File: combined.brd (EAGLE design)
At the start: 179 x 79.7 mm, 201 parts, among them U1 LM4562MAX/NOPB, U10 LM4562MAX/NOPB, U11 LM4562MAX/NOPB, U12 MAX5419LETA+, U13 MAX5419LETA+, U14 LM4562MAX/NOPB, U15 LM4562MAX/NOPB, U16 LM4562MAX/NOPB, U17 LM4562MAX/NOPB, U2 LM4562MAX/NOPB, U3 LM4562MAX/NOPB, U4 LM4562MAX/NOPB, U5 LM4562MAX/NOPB, U6 MAX5419LETA+, U7 MAX5419LETA+, U8 LM4562MAX/NOPB, U9 LM4562MAX/NOPB

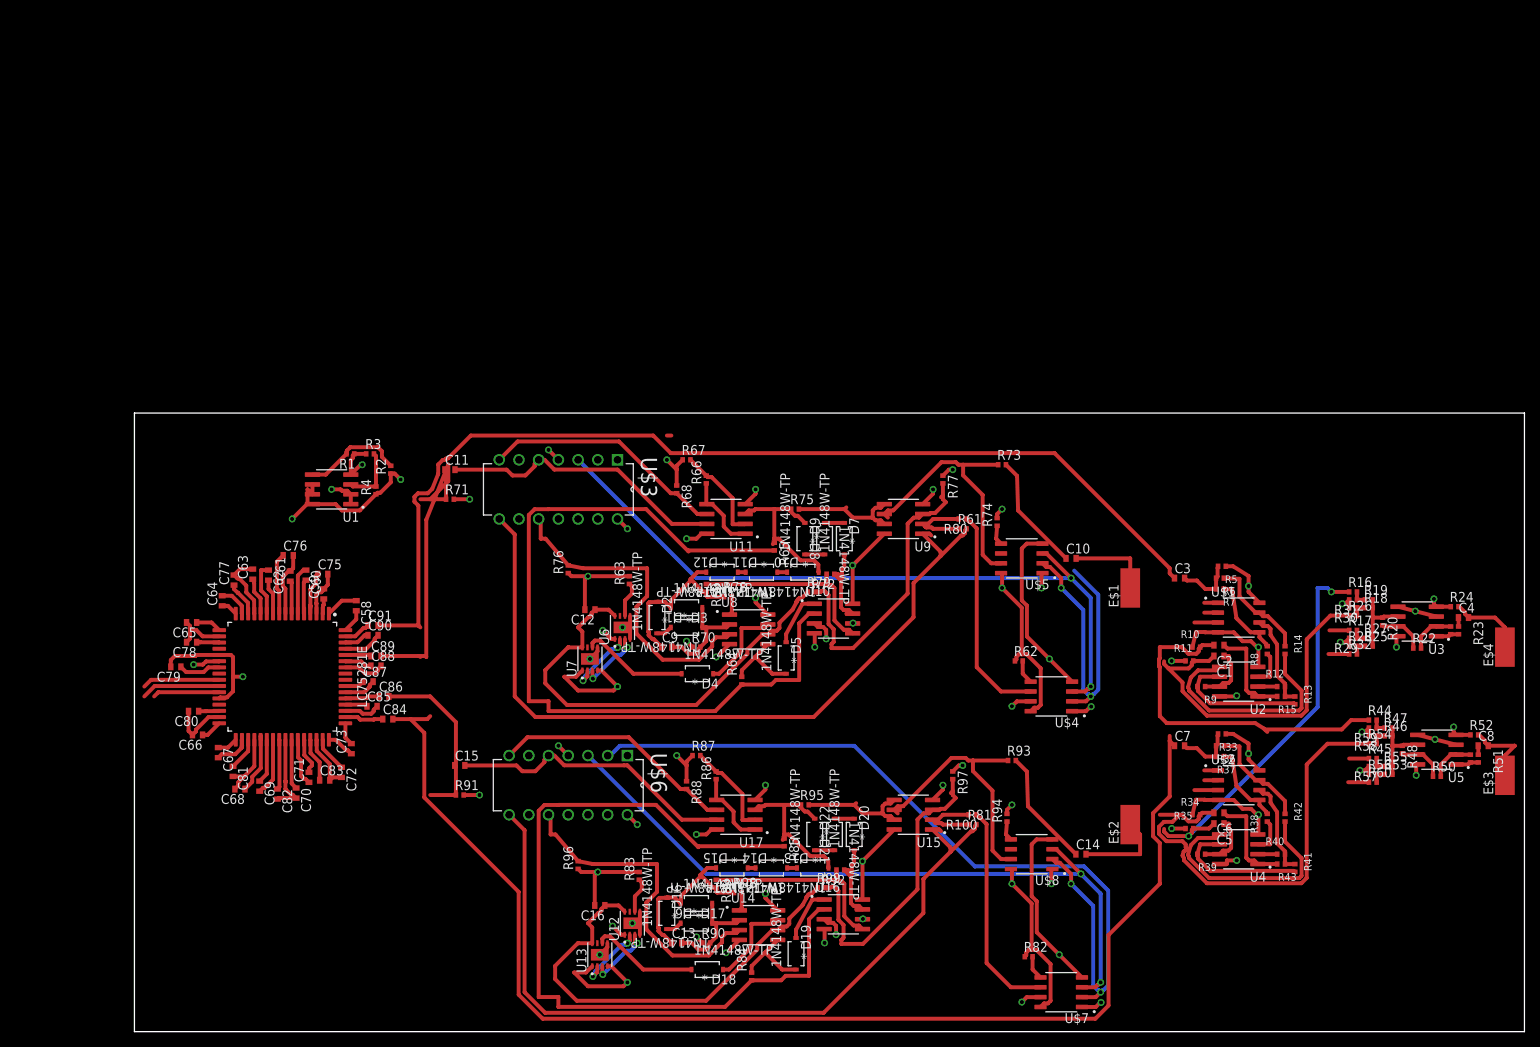
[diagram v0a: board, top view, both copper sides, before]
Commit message: corrections
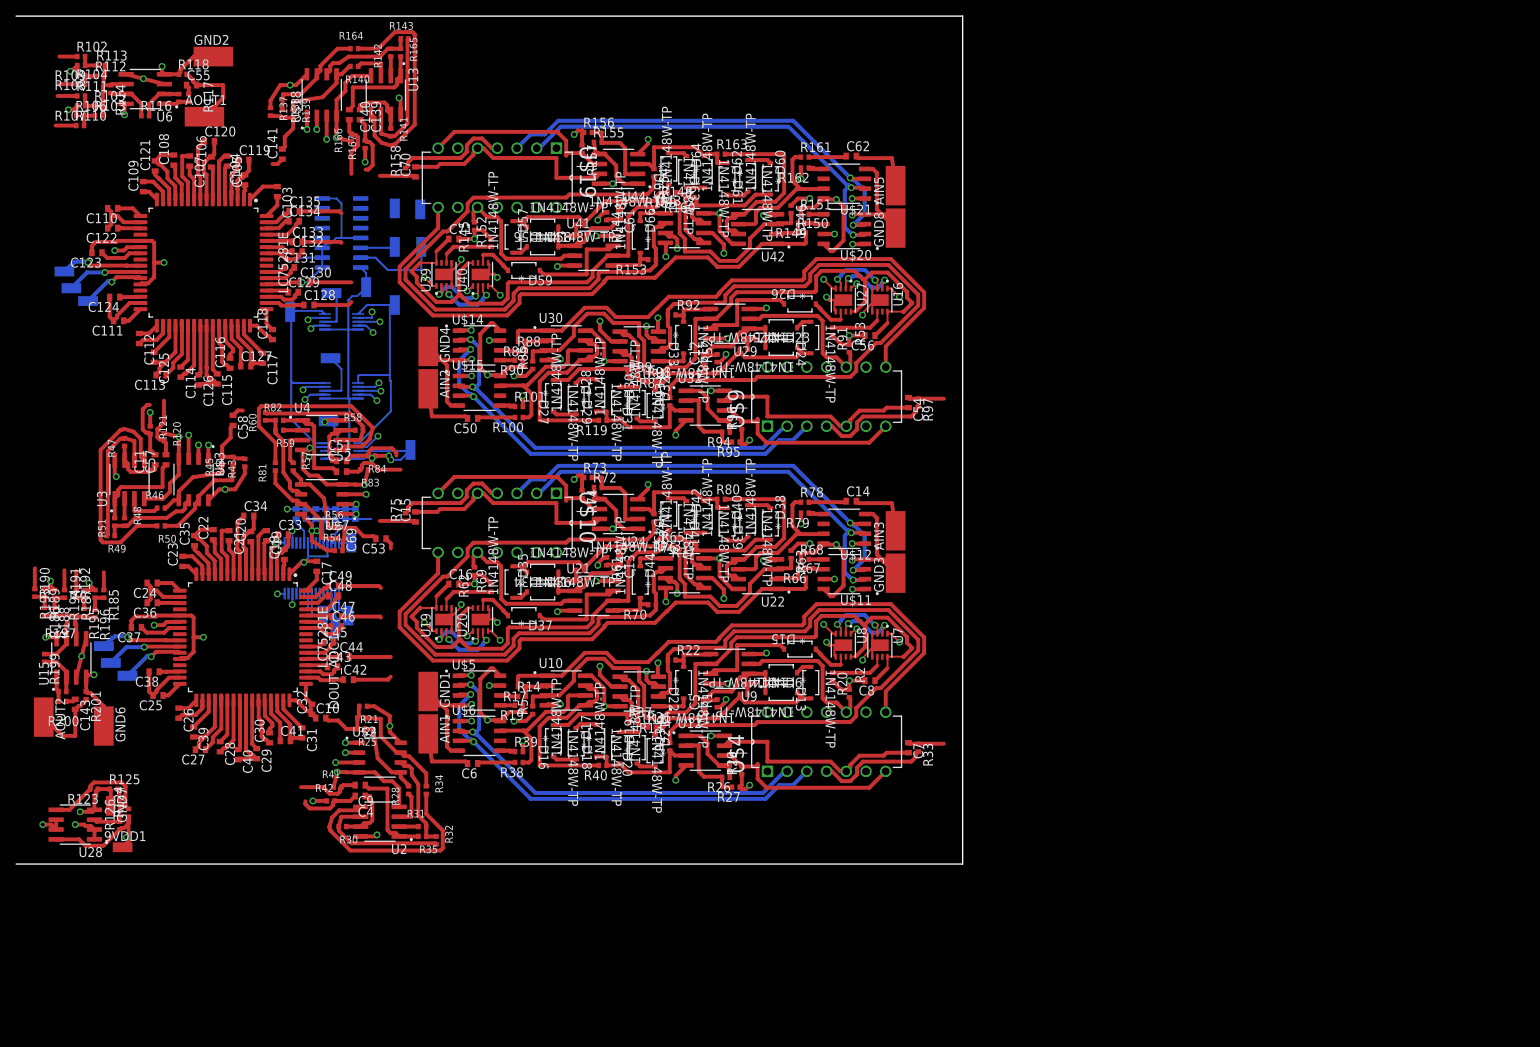
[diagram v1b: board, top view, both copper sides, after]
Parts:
- removed C1, C2, C3: 0.1u, rcl:C0402
- removed C59, C60, C72, C73: 0.047uF, rcl:C0402
- removed C75, C76, C77, C78, C79, C80, C81, C82, C83, C84, C85, C86, C87, C88, C89, C90, C91: 10uF, rcl:C0402
- removed D1, D10, D11, D12, D2, D3, D4, D5, D7, D8, D9: 1N4148W-TP, 1N4148W-TP:SOD123
- removed E$1, E$2, E$3, E$4: (no value), wirepad:SMD2,54-5,08
- removed R10, R11: 1.5M, rcl:R0402
- removed R15, R18, R9: 20k, rcl:R0402
- removed R16: 5k, rcl:R0402
- removed R3: 1k, rcl:R0402
- removed R4: 1.7k, rcl:R0402
- removed R6, R7: 10k, rcl:R0402
- removed R8: 4k, rcl:R0402
- removed U$1, U$8: MCP4131-503E/SN, MCP4131-503E_SN:SOIC127P599X175-8N
- removed U1, U14, U5: LM4562MAX/NOPB, LM4562MAX_NOPB:SOIC127P599X175-8N
- added 3V3_D1, 9VDD1, BCK_ADC1, CE_EQ1, CE_EQ2, CLK_ADC1, CL_EQ1, CL_EQ2, CS3, CS4, CS5, DI_EQ1, DI_EQ2, DOUT_ADC1, GND5, GND7, LRCK_ADC1, MUX2, MUX3, SCK1, SCL1, SDA1, SDI/O1: (no value), wirepad:SMD1,27-2,54
- added AIN1, AIN2, AIN3, AIN5, AOUT1, AOUT2, GND1, GND2, GND3, GND4, GND6, GND8: (no value), wirepad:SMD2,54-5,08
- added C103, C104, C105, C106, C107, C108, C109, C110, C111, C112, C113, C114, C115, C116, C117, C118, C17, C18, C19, C20, C21, C22, C23, C24, C25, C26, C27, C28, C29, C30, C31, C32: 0.047uF, rcl:C0402
- added C119, C120, C121, C122, C123, C124, C125, C126, C127, C128, C129, C130, C131, C132, C133, C134, C135, C33, C34, C35, C36, C37, C38, C39, C40, C41, C42, C43, C44, C45, C46, C47, C48, C49: 10uF, rcl:C0402
- added C139, C140, C141, C143, C51, C52, C53, C55, C57: 0.1u, rcl:C0402
- added C50: 0.1, rcl:C0402
- added C54, C56: 1.5u, rcl:C0402
- added D23, D24, D25, D26, D27, D28, D29, D30, D31, D32, D33, D34, D35, D36, D37, D38, D39, D40, D41, D42, D43, D44, D56, D57, D58, D59, D60, D61, D62, D63, D64, D65, D66: 1N4148W-TP, 1N4148W-TP:SOD123
- added IC2: PCM1865DBT, PCM1865DBT:TSSOP-30
- added R101, R137, R138, R139, R145, R151, R156, R162: 10k, rcl:R0402
- added R102, R104, R106, R107, R108, R109, R110, R111, R185, R187, R189, R190, R191, R192, R193, R194: 5k, rcl:R0402
- added R103, R105, R112, R113, R114, R115, R116, R141, R157, R165, R186, R188, R195, R196, R197, R198, R199: 20k, rcl:R0402
- added R117, R123, R124, R125, R147, R200: 1k, rcl:R0402
- added R118, R120, R121, R166, R167, R201: 1.5M, rcl:R0402
- added R119, R144, R149, R150, R152, R153, R154, R155, R159, R160, R161, R163: 100k, rcl:R0402
- added R126: 1.7k, rcl:R0402
- added R140, R164: 4k, rcl:R0402
- added R142, R143: 6k, rcl:R0402
- added R146, R148: 470k, rcl:R0402
- added R158: 1M, rcl:R0402
- added U$10, U$19, U$9: MCP42100-I/P, MCP42100-I_P:DIP254P762X432-14
- added U$11, U$12, U$15, U$18, U$20, U$21: MCP4131-503E/SN, MCP4131-503E_SN:SOIC127P599X175-8N
- added U$13, U$16: LC75281E, LC75281E:QFP80P1720X1720X270-64N
- added U18, U25: TMUX1204DGSR, TMUX1204DGSR:SOP50P490X110-10N
- added U19, U20, U27, U39, U40: MAX5419LETA+, MAX5419LETA_:SON65P300X300X80-9N
- added U21, U22, U23, U24, U28, U29, U30, U31, U32, U41, U42, U43, U44: LM4562MAX/NOPB, LM4562MAX_NOPB:SOIC127P599X175-8N
- added U26: TCA9546ADR, TCA9546ADR:SOIC127P600X175-16N
- C10: value 0.1 -> 0.1u
- C11: value 1.5u -> 0.1u
- C12: value 1.5u -> 680p
- C5: value 0.1u -> 680p
- C58: value 0.047uF -> 0.1u
- C6: value 0.1u -> 0.1
- C61: value 0.047uF -> 680p
- C62: value 0.047uF -> 0.1
- C63, C65, C68: value 0.047uF -> 0.1μF
- C64, C66: value 0.047uF -> 10μF
- C67, C69: value 0.047uF -> 1μF
- C7, C8: value 0.1u -> 1.5u
- C70, C71: value 0.047uF -> 1.5u
- C9: value 680p -> 0.1u
- R1, R23, R78, R98: value 1k -> 100k
- R12: value 6k -> 1k
- R13: value 6k -> 470k
- R14, R38: value 4k -> 100k
- R17, R26: value 5k -> 100k
- R19, R21, R25, R27, R39, R43, R53, R55, R68: value 20k -> 10k
- R2: value 1k -> 10k
- R20, R22, R88: value 20k -> 100k
- R24: value 1.5M -> 10k
- R28, R57: value 5k -> 4k
- R29, R30, R58: value 5k -> 20k
- R31, R32, R59, R60: value 5k -> 6k
- R33: value 10k -> 1M
- R34: value 1.5M -> 4k
- R35: value 1.5M -> 20k
- R36, R37, R67, R76, R94: value 10k -> 100k
- R40: value 6k -> 100k
- R41: value 6k -> 1.5M
- R42: value 4k -> 1.5M
- R44, R45, R54, R56: value 5k -> 10k
- R46, R50: value 20k -> 4k
- R48, R49: value 20k -> 6k
- R5, R87: value 10k -> 470k
- R51: value 1k -> 20k
- R52: value 1.5M -> 100k
- R63, R65, R85: value 100k -> 470k
- R64, R86: value 100k -> 1k
- R71, R91: value 1M -> 100k
- R73, R90, R95: value 100k -> 10k
- R74, R82, R96: value 10k -> 20k
- R75: value 100k -> 1M
- R77, R99: value 470k -> 100k
- R79: value 470k -> 10k
- R81: value 100k -> 4k
- R83, R84: value 100k -> 1.5M
- R97: value 470k -> 1M
- U$14: value LC75281E -> MCP4131-503E/SN; device LC75281E:QFP80P1720X1720X270-64N -> MCP4131-503E_SN:SOIC127P599X175-8N
- U$3, U$6: value MCP42100-I/P -> MCP4131-503E/SN; device MCP42100-I_P:DIP254P762X432-14 -> MCP4131-503E_SN:SOIC127P599X175-8N
- U$4: value MCP4131-503E/SN -> MCP42100-I/P; device MCP4131-503E_SN:SOIC127P599X175-8N -> MCP42100-I_P:DIP254P762X432-14
- U12, U13, U6: value MAX5419LETA+ -> LM4562MAX/NOPB; device MAX5419LETA_:SON65P300X300X80-9N -> LM4562MAX_NOPB:SOIC127P599X175-8N
- U16, U8: value LM4562MAX/NOPB -> MAX5419LETA+; device LM4562MAX_NOPB:SOIC127P599X175-8N -> MAX5419LETA_:SON65P300X300X80-9N
- U17: value LM4562MAX/NOPB -> TMUX1204DGSR; device LM4562MAX_NOPB:SOIC127P599X175-8N -> TMUX1204DGSR:SOP50P490X110-10N
- moved R51 178.3 mm to (12.7, 44.1)
- moved R49 177.5 mm to (12.2, 42.3), turned to 180 degrees
- moved R50 167.5 mm to (18.7, 43.6), turned to 180 degrees
- moved R48 167.2 mm to (14.0, 44.1)
- moved R47 166.9 mm to (14.0, 54.4), turned to 90 degrees
- moved U3 166.9 mm to (14.6, 49.5), turned to 90 degrees
- moved R46 160.8 mm to (18.7, 45.8)
- moved R45 153.1 mm to (26.5, 51.9), turned to 90 degrees
- moved R44 150.6 mm to (27.9, 51.9), turned to 90 degrees
- moved R60 150.2 mm to (32.1, 57.7), turned to 90 degrees
- moved R59 146.0 mm to (33.9, 55.9)
- moved R57 144.3 mm to (35.7, 51.2), turned to 270 degrees
- moved C4 144.0 mm to (44.3, 8.76), turned to 180 degrees
- moved R43 143.1 mm to (29.5, 51.7), turned to 90 degrees
- moved R24 141.6 mm to (44.5, 18.8), turned to 180 degrees
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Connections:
- removed net CS5: U$7.1
- removed net CS6: U$8.1
- removed net EQ1_CE: U$14.27
- removed net EQ1_CL: U$14.25
- removed net EQ1_DI: U$14.26
- removed net H_1: C16.1, R99.1, U12.8, U13.8, U14.6
- removed net L_2: R83.1, U12.6
- removed net L_3: D18.C, U13.6
- removed net N$12: R21.2, R23.1, U3.1
- removed net N$123: C58.1, U$14.1
- removed net N$125: C60.1, U$14.6
- removed net N$126: C61.1, U$14.7
- removed net N$127: C62.1, U$14.11
- removed net N$128: C63.1, U$14.12
- removed net N$129: C64.1, U$14.16
- removed net N$130: C65.1, U$14.17
- removed net N$134: C67.1, U$14.33
- removed net N$180: C68.1, U$14.37
- removed net N$183: C71.1, U$14.43
- removed net N$184: C72.1, U$14.47
- removed net N$185: C73.1, U$14.48
- removed net N$186: C58.2, U$14.64
- removed net N$187: C59.2, C75.2, U$14.3
- removed net N$188: C75.1, U$14.4
- removed net N$189: C76.1, U$14.9
- removed net N$190: C77.1, U$14.14
- removed net N$192: C79.1, U$14.23
- removed net N$193: C80.1, U$14.30
- removed net N$194: C81.1, U$14.35
- removed net N$195: C82.1, U$14.40
- removed net N$196: C83.1, U$14.45
- removed net N$197: C84.1, U$14.50
- removed net N$198: C85.1, U$14.52
- removed net N$199: C86.1, U$14.53
- removed net N$200: C87.1, U$14.55
- removed net N$201: C88.1, U$14.59
- removed net N$202: C89.1, U$14.60
- removed net N$203: C90.1, U$14.62
- removed net N$204: C91.1, U$14.63
- removed net N$205: C60.2, U$14.5
- removed net N$206: C61.2, C76.2, U$14.8
- removed net N$207: C62.2, U$14.10
- removed net N$208: C63.2, C77.2, U$14.13
- removed net N$209: C64.2, U$14.15
- removed net N$210: C65.2, C78.2, U$14.18
- removed net N$212: C67.2, U$14.34
- removed net N$214: C69.2, U$14.39
- removed net N$215: C70.2, C82.2, U$14.41
- removed net N$216: C71.2, U$14.44
- removed net N$217: C72.2, C83.2, U$14.46
- removed net N$218: C73.2, U$14.49
- removed net N$219: C85.2, U$14.51
- removed net N$222: C88.2, U$14.58
- removed net N$224: C90.2, U$14.61
- removed net N$24: R42.2, U4.5
- removed net N$25: R38.1, U4.3
- removed net N$32: R46.2, R47.2, R48.1, R53.2, R55.2, U5.6
- removed net N$5 (its old number): R8.1, U2.3
- removed net P0A_2: R82.2, U$7.5
- removed net P0A_3: R94.1, U$8.5
- removed net P0B_2: R93.1, U$8.7, U15.6
- removed net P0W_1: R100.1, U$7.6
- removed net PA2: R81.2, U$6.8, U15.1
- removed net PA3: R88.2, U$6.7, U17.6
- removed net PB2: R96.2, U$6.10, U14.3
- removed net PB3: C15.2, U$6.5, U17.7
- removed net S$1: U$4.2, U$5.2
- removed net S$2: U$3.2
- removed net S$4: U1.6, U1.7
- removed net S$5: R2.1, R4.1, U1.8
- removed net SCK1: U$2.2
- removed net SCK2: U$6.2, U$7.2, U$8.2
- removed net SCL1: U12.2, U13.2
- removed net SDA1: U12.3, U13.3
- removed net SDI/O1: U$2.3
- removed net SDI/O2: U$3.3, U$4.3, U$5.3
- removed net SDI/O3: U$6.3, U$7.3, U$8.3
- removed net VDD1: R62.1, U$3.14, U$4.8, U$5.8, U10.8, U11.8, U6.1, U7.1, U7.4, U8.8, U9.8
- removed net VDD2: R82.1, U$6.14, U$7.8, U$8.8, U12.1, U13.1, U13.4, U14.8, U15.8, U16.8, U17.8
- removed net VREF1: C12.2, R63.2, R67.1, R68.1, R70.1, R74.2, R76.1, R77.1, U$4.7, U10.3, U10.6
- removed net VREF2: C16.2, R83.2, R87.1, R88.1, R90.1, R94.2, R96.1, R97.1, U$7.7, U16.3, U16.6
- removed net VSS1: R91.2, U$6.4, U$7.4, U$8.4, U12.4, U12.5, U12.9, U13.5, U13.9, U14.4, U15.4, U16.4, U17.4
- new net +3V3: 3V3_D1.1, U17.5, U17.6, U18.5, U18.6, U25.5, U25.6, U26.16
- new net 3V3D: C63.1, C64.1, IC2.13, IC2.14
- new net AIN01: R110.1
- new net AIN02: R193.1
- new net AIN11: R111.1
- new net AIN12: C53.1
- new net AIN123: R194.1
- new net AIN223: R187.1
- new net AIN31: C141.1
- new net AIN323: R185.1
- new net AIN33: AIN2.1, C50.2
- new net AIN45: C58.1
- new net AOUT2: C15.1, R75.1
- new net AOUT23: AOUT2.1, C143.2, R201.2
- new net AOUT3: C54.1, R97.1
- new net AOUT4: C70.1, R158.1
- new net AOUTL3: C140.2, R166.2
- new net AOUTL4: C57.2, R120.2
- new net AOUTR3: C139.2, R167.2
- new net AOUTR4: C11.2, R121.2
- new net BCK_ADC: BCK_ADC1.1, IC2.17
- new net CLK_ADC: CLK_ADC1.1, IC2.15
- new net CS01: U$10.1
- new net CS03: U$9.1
- new net CS04: U$19.1
- new net CS0D: CS3.1, U17.8
- new net CS0_0: U17.2
- new net CS0_1: U17.9
- new net CS0_2: U17.4
- new net CS0_3: U17.7
- new net CS11: U$11.1
- new net CS13: U$14.1
- new net CS14: U$20.1
- new net CS1D: CS4.1, U25.8
- new net CS1_0: U25.2
- new net CS1_1: U25.9
- new net CS1_2: U25.4
- new net CS1_3: U25.7
- new net CS21: U$12.1
- new net CS23: U$15.1
- new net CS24: U$21.1
- new net CS2D: CS5.1, U18.8
- new net CS2_0: U18.2
- new net CS2_1: U18.9
- new net CS2_2: U18.4
- new net CS2_3: U18.7
- new net DGND: GND5.1, U17.3, U18.3, U25.3, U26.1, U26.13, U26.2, U26.3, U26.8
- new net DOUT_ADC: DOUT_ADC1.1, IC2.18
- new net EIN01: C130.2
- new net EIN11: C133.2
- new net EOUT01: C128.2
- new net EOUT11: C135.2
- new net EQ1_CE1: CE_EQ1.1, U$13.27
- new net EQ1_CE2: CE_EQ2.1, U$16.27
- new net EQ1_CL1: CL_EQ1.1, U$13.25
- new net EQ1_CL2: CL_EQ2.1, U$16.25
- new net EQ1_DI1: DI_EQ1.1, U$13.26
- new net EQ1_DI2: DI_EQ2.1, U$16.26
- new net H_01: C16.1, R65.1, U19.8, U20.8, U21.6
- new net H_03: C56.1, R87.1, U16.8, U27.8, U29.6
- new net H_04: C71.1, R148.1, U39.8, U40.8, U41.6
- new net LRCK_ADC: IC2.16, LRCK_ADC1.1
- new net L_01: R69.1, U19.6
- new net L_03: R91.1, U16.6
- new net L_04: R152.1, U39.6
- new net L_11: D37.C, U20.6
- new net L_13: D26.C, U27.6
- new net L_14: D59.C, U40.6
- new net MUX0: MUX2.1, U17.1, U18.1, U25.1
- new net MUX1: MUX3.1, U17.10, U18.10, U25.10
- new net N$100: C105.1, U$16.6
- new net N$101: C106.1, U$16.7
- new net N$102: D56.A, D57.C
- new net N$103: D61.A, D62.C
- new net N$104: D60.A, D61.C
- new net N$105: C62.1, R161.2
- new net N$106: D64.A, D65.C
- new net N$107: D63.A, D64.C
- new net N$108: C107.1, U$16.11
- new net N$109: C108.1, U$16.12
- new net N$110: C109.1, U$16.16
- new net N$111: C110.1, U$16.17
- new net N$112: C111.1, U$16.32
- new net N$113: C112.1, U$16.33
- new net N$114: C113.1, U$16.37
- new net N$115: C114.1, U$16.38
- new net N$116: C115.1, U$16.42
- new net N$117: C116.1, U$16.43
- new net N$118: C117.1, U$16.47
- new net N$119: C118.1, U$16.48
- new net N$120: C103.2, U$16.64
- new net N$121: C104.2, C119.2, U$16.3
- new net N$122: C119.1, U$16.4
- new net N$124: C120.1, U$16.9
- new net N$131: C121.1, U$16.14
- new net N$132: C122.1, U$16.19
- new net N$135: C123.1, U$16.23
- new net N$136: C124.1, U$16.30
- new net N$137: C125.1, U$16.35
- new net N$138: C126.1, U$16.40
- new net N$139: C127.1, U$16.45
- new net N$140: C128.1, U$16.50
- new net N$141: D37.A, U21.7
- new net N$1413: R103.2, R105.2, R112.2, R113.2, R114.1, U6.6
- new net N$142: D39.A, D40.C
- new net N$1421: R186.2, R188.2, R195.2, R196.2, R197.1, U15.6
- new net N$143: C129.1, U$16.52
- new net N$1433: D26.A, U29.7
- new net N$144: R147.2, U41.1
- new net N$1444: D59.A, U41.7
- new net N$145: C130.1, U$16.53
- new net N$146: C131.1, U$16.55
- new net N$147: C132.1, U$16.59
- new net N$148: C133.1, U$16.60
- new net N$149: C134.1, U$16.62
- new net N$150: C135.1, U$16.63
- new net N$151: D44.C, R70.2, U21.5
- new net N$152: D38.A, D39.C
- new net N$153: C105.2, U$16.5
- new net N$1533: D33.C, R92.2, U29.5
- new net N$154: C106.2, C120.2, U$16.8
- new net N$1544: D66.C, R153.2, U41.5
- new net N$155: C107.2, U$16.10
- new net N$156: C108.2, C121.2, U$16.13
- new net N$157: C109.2, U$16.15
- new net N$158: C110.2, C122.2, U$16.18
- new net N$159: C111.2, C124.2, U$16.31
- new net N$160: C112.2, U$16.34
- new net N$161: R70.1, R71.2, U23.2
- new net N$162: C14.1, R78.2
- new net N$163: C113.2, C125.2, U$16.36
- new net N$1633: R92.1, R93.2, U31.2
- new net N$164: C114.2, U$16.39
- new net N$1644: R153.1, R154.2, U43.2
- new net N$165: C115.2, C126.2, U$16.41
- new net N$166: C116.2, U$16.44
- new net N$167: C117.2, C127.2, U$16.46
- new net N$168: C118.2, U$16.49
- new net N$169: C129.2, U$16.51
- new net N$170: C131.2, U$16.54
- new net N$171: C132.2, U$16.58
- new net N$172: C134.2, U$16.61
- new net N$173: C104.1, U$16.2
- new net N$175: C141.2, R137.2, R138.2, R139.2
- new net N$1833: R94.1, U32.1, U32.5
- new net N$1844: R155.1, U44.1, U44.5
- new net N$1933: R94.2, R95.2, U32.2
- new net N$1944: R155.2, R156.2, U44.2
- new net N$2012: C53.2, R54.2, R55.2, R56.2
- new net N$2111: C13.1, D35.A, D36.C, D43.A, R64.1, R76.2
- new net N$21111: C17.1, U$13.1
- new net N$2133: C12.1, D24.A, D25.C, D32.A, R86.1, R98.2
- new net N$2144: C61.1, D57.A, D58.C, D65.A, R147.1, R159.2
- new net N$223: C143.1, R200.2
- new net N$225: R186.1, R189.2, R193.2
- new net N$226: R185.2, R192.1, R196.1
- new net N$227: R187.2, R191.1, R195.1
- new net N$228: R188.1, R190.1, R194.2
- new net N$233: D27.C, R99.1, U31.7
- new net N$244: D60.C, R160.1, U43.7
- new net N$246: D62.A, D63.C, R154.1, R163.1, U44.3
- new net N$261: D40.A, D41.C, R71.1, R80.1, U24.3
- new net N$2611: C21.1, U$13.11
- new net N$2633: D29.A, D30.C, R119.1, R93.1, U32.3
- new net N$271: R80.2, U22.5, U22.7
- new net N$2711: C22.1, U$13.12
- new net N$2733: R119.2, U30.5, U30.7
- new net N$2744: R163.2, U42.5, U42.7
- new net N$312: R81.2, U4.5
- new net N$331: R164.2, U13.5
- new net N$333: C12.2, D23.C, D25.A, R52.2, U29.2
- new net N$344: C61.2, D56.C, D58.A, R144.2, U41.2
- new net N$411: C17.2, U$13.64
- new net N$413: R114.2, R116.1, U6.7
- new net N$414: R50.2, U3.5
- new net N$421: R197.2, R199.1, U15.7
- new net N$433: D33.A, U31.1
- new net N$444: D66.A, U43.1
- new net N$500: R28.1, U2.3
- new net N$512: R57.1, U4.3
- new net N$513: R115.1, R116.2, U6.2
- new net N$514: R46.1, U3.3
- new net N$521: R198.1, R199.2, U15.2
- new net N$531: R140.1, U13.3
- new net N$600: R31.1, U2.2
- new net N$611: C20.2, C34.2, U$13.8
- new net N$612: R59.1, U4.2
- new net N$614: R48.1, U3.2
- new net N$631: R142.1, U13.2
- new net N$633: R85.2, R87.2, U30.3
- new net N$644: R146.2, R148.2, U42.3
- new net N$68: C27.2, C39.2, U$13.36
- new net N$700: R30.2, R32.2, U2.6
- new net N$711: C30.2, U$13.44
- new net N$712: R58.2, R60.2, U4.6
- new net N$714: R47.2, R49.2, U3.6
- new net N$731: R141.2, R143.2, U13.6
- new net N$733: R88.2, R89.1, U30.2
- new net N$744: R149.2, R150.1, U42.2
- new net N$78: C18.1, U$13.2
- new net N$80: C55.1, R117.2
- new net N$800: C4.1, R30.1, U2.7
- new net N$81: R76.1, R77.2, U23.5
- new net N$812: C51.1, R58.1, U4.7
- new net N$814: C11.1, R47.1, U3.7
- new net N$82: R103.1, R106.2, R110.2
- new net N$83: R102.2, R109.1, R113.1
- new net N$831: C139.1, R141.1, U13.7
- new net N$833: R98.1, R99.2, U31.5
- new net N$84: R104.2, R108.1, R112.1
- new net N$844: R159.1, R160.2, U43.5
- new net N$85: R105.1, R107.1, R111.2
- new net N$86: D23.A, D24.C
- new net N$87: D28.A, D29.C
- new net N$88: C67.1, IC2.6
- new net N$89: C68.1, C69.1, IC2.11
- new net N$90: D27.A, D28.C
- new net N$91: C50.1, R100.2
- new net N$912: C52.1, R82.2, U4.1
- new net N$914: C57.1, R51.2, U3.1
- new net N$92: R125.2, R126.2, U28.3
- new net N$93: R123.2, R124.2, U28.5
- new net N$931: C140.1, R165.2, U13.1
- new net N$94: D31.A, D32.C
- new net N$95: D30.A, D31.C
- new net N$99: C103.1, U$16.1
- new net P0A31: R139.1, R140.2, U$18.5
- new net P0A4: R45.1, R46.2, U$3.5
- new net P0A_01: R68.2, U$11.5
- new net P0A_03: R90.2, U$14.5
- new net P0A_04: R151.2, U$20.5
- new net P0A_11: R79.1, U$12.5
- new net P0A_13: R101.1, U$15.5
- new net P0A_14: R162.1, U$21.5
- new net P0B31: R138.1, R164.1, U$18.7
- new net P0B4: R44.1, R50.1, U$3.7
- new net P0B_11: R78.1, U$12.7, U22.6
- new net P0B_13: R100.1, U$15.7, U30.6
- new net P0B_14: R161.1, U$21.7, U42.6
- new net P0W31: R142.2, R143.1, R165.1, U$18.6
- new net P0W4: R48.2, R49.1, R51.1, U$3.6
- new net P0W_01: R66.1, U$11.6
- new net P0W_03: R88.1, U$14.6
- new net P0W_04: R149.1, U$20.6
- new net PA01: R67.2, U$10.8, U22.1
- new net PA03: R89.2, U$9.8, U30.1
- new net PA04: R150.2, U$19.8, U42.1
- new net PA11: R74.2, U$10.7, U24.6
- new net PA13: R96.2, U$9.7, U32.6
- new net PA14: R157.2, U$19.7, U44.6
- new net PB01: R62.2, U$10.10, U21.3
- new net PB03: R53.2, U$9.10, U29.3
- new net PB04: R145.2, U$19.10, U41.3
- new net PB11: C15.2, U$10.5, U24.7
- new net PB13: C54.2, U$9.5, U32.7
- new net PB14: C70.2, U$19.5, U44.7
- new net RS3: U$9.11
- new net RS4: U$19.11
- new net SCL_0: U26.5
- new net SCL_1: U26.4
- new net SCL_2: U26.10
- new net SCL_3: U26.9
- new net SDA_0: U26.7
- new net SDA_1: U26.6
- new net SDA_2: U26.12
- new net SDA_3: U26.11
- new net SHDN3: U$9.12
- new net SHDN4: U$19.12
- new net VIN1: IC2.1
- new net VIN2: IC2.3
- new net VIN3: IC2.30
- new net VIN4: IC2.28
- net 3V3A: now also C65.1, C66.1, IC2.8, U28.1, U28.2; no longer U1.1, U1.2
- net AIN: now also AIN1.1, C6.2; no longer C10.2, E$1.1
- net AIN0: now also C10.1; no longer R32.1
- net AIN1: now also AIN3.1, C14.2; no longer R17.1
- net AIN2: now also R104.1; no longer C14.2, E$2.1
- net AIN3: now also R102.1; no longer R60.1
- net AIN4: now also AIN5.1, C62.2; no longer R45.1
- net AOUT: now also C7.1, R33.1; no longer C4.2, E$4.1, R24.2
- net AOUT1: now also AOUT1.1, C55.2, R118.2; no longer C8.2, E$3.1, R52.2
- net AOUTL: now also C9.2, R41.2; no longer C2.2, R10.2, R44.1
- net AOUTL1: now also C52.2, R83.2; no longer C6.2, R34.2, R54.1
- net AOUTR: now also C4.2, R42.2; no longer C1.2, R11.2, R26.1
- net AOUTR1: now also C51.2, R84.2; no longer C5.2, R16.1, R35.2
- net CS: now also U$2.1; no longer U$1.1
- net CS0: now also U$4.1; no longer U$3.1
- net CS1: now also U$5.1, U$7.1; no longer U$2.1
- net CS2: now also U$6.1; no longer U$4.1
- net CS3: now also U$18.1; no longer U$5.1
- net CS4: now also U$3.1; no longer U$6.1
- net EIN0: now also C44.2; no longer C15.1, C86.2, R91.1
- net EIN1: now also C47.2; no longer C11.1, C89.2, R71.1
- net EOUT0: now also C42.2; no longer C7.1, C84.2
- net EOUT1: now also C49.2; no longer C3.1, C91.2
- net GND: now also C123.2, C37.2, C63.2, C64.2, C65.2, C66.2, C67.2, C68.2, C69.2, GND2.1, GND6.1, GND7.1, IC2.12, IC2.7, R118.1, R120.1, R121.1, R123.1, R125.1, R166.1, R167.1, R201.1, R41.1, R42.1, R83.1, R84.1, U$13.21, U$13.28, U$16.21, U$16.28, U$18.4, U$3.4, U$7.4, U13.4, U15.4, U28.4, U6.4; no longer C79.2, R1.1, R10.1, R11.1, R24.1, R3.1, R34.1, R35.1, R52.1, U$1.4, U$14.21, U$14.28, U1.4, U5.4
- net H_0: now also C8.1, R13.1, U8.8, U9.6; no longer C12.1, R79.1, U6.8, U8.6
- net L_0: now also R20.1, U7.6; no longer R63.1, U6.6
- net L_1: now also D15.C, U8.6; no longer D4.C, U7.6
- net N$1: now also D13.C, D6.A, R12.2, U9.1; no longer R3.2, R4.2, U1.3
- net N$10: now also C10.2, R21.2, R24.2, R25.2; no longer C59.1, U$14.2
- net N$11: now also R64.2, U21.1; no longer C4.1, R23.2
- net N$13: now also D34.A, D35.C; no longer R20.2, R22.1, U3.7
- net N$133: now also R86.2, U29.1; no longer C66.1, U$14.32
- net N$14: now also D15.A, U9.7; no longer R21.1, R22.2, U3.2
- net N$15: now also D22.C, R22.2, U9.5; no longer R25.1, R28.2, R32.2
- net N$16: now also R22.1, R23.2, U11.2; no longer R18.2, R19.2, R20.1, R25.2, R27.2, U3.6
- net N$17: now also D42.A, D43.C; no longer R16.2, R19.1, R31.1
- net N$18: now also R26.1, U12.1, U12.5; no longer R18.1, R26.2, R30.1
- net N$181: now also R72.1, U24.1, U24.5; no longer C69.1, U$14.38
- net N$182: now also D41.A, D42.C; no longer C70.1, U$14.42
- net N$19: now also R26.2, R27.2, U12.2; no longer R17.2, R27.1, R29.1
- net N$191: now also R72.2, R73.2, U24.2; no longer C78.1, U$14.19
- net N$2: now also D16.C, D17.A, D18.C, R37.1, U11.7; no longer R1.2, R2.2, U1.5
- net N$20: now also C58.2, R43.2, R44.2, R45.2; no longer C7.2, R33.2, R36.2, R37.2
- net N$21: now also C5.1, D13.A, D14.C, D21.A, R12.1, R36.2; no longer R39.2, R41.2, U4.6
- net N$211: now also D38.C, R77.1, U23.7; no longer C66.2, C80.2, U$14.31
- net N$213: now also R115.2, R117.1, U6.1; no longer C68.2, C81.2, U$14.36
- net N$22: now also C19.1, U$13.6; no longer C5.1, R39.1, U4.7
- net N$221: now also R198.2, R200.1, U15.1; no longer C87.2, U$14.54
- net N$23: now also C20.1, U$13.7; no longer C6.1, R43.2, U4.1
- net N$26: now also D18.A, D19.C, R23.1, U12.3; no longer U4.2
- net N$27: now also R40.2, U10.5, U10.7; no longer C8.1, R51.2
- net N$28: now also C23.1, U$13.16; no longer R49.2, R51.1, U5.1
- net N$29: now also C24.1, U$13.17; no longer R48.2, R50.1, U5.7
- net N$3: now also C5.2, D14.A, D16.A, D17.C, D6.C, R1.2, U9.2; no longer C3.2, R5.2, R6.2, R7.2
- net N$30: now also R34.2, U2.5; no longer R49.1, R50.2, U5.2
- net N$31: now also C13.2, D34.C, D36.A, R61.2, U21.2; no longer R53.1, R56.2, R60.2
- net N$33: now also C25.1, U$13.32; no longer R44.2, R47.1, R59.1
- net N$34: now also C26.1, U$13.33; no longer R46.1, R54.2, R58.1
- net N$35: now also C27.1, U$13.37; no longer R45.2, R55.1, R57.1
- net N$36: now also C28.1, U$13.38; no longer C9.2, D1.C, D3.A, R70.2, U8.2
- net N$37: now also C29.1, U$13.42; no longer R77.2, R79.2, U9.3
- net N$38: now also C30.1, U$13.43; no longer R61.1, R80.2, U9.2
- net N$39: now also C31.1, U$13.47; no longer D5.C, R64.2, U8.5
- net N$4: now also C6.1, D22.A, R38.2, U11.1; no longer R14.2, U2.5
- net N$40: now also C32.1, U$13.48; no longer R64.1, R65.2, U10.2
- net N$41: now also D44.A, U23.1; no longer R66.1, U11.1, U11.5
- net N$42: now also C18.2, C33.2, U$13.3; no longer R66.2, R67.2, U11.2
- net N$43: now also C33.1, U$13.4; no longer D1.A, D2.C
- net N$44: now also C34.1, U$13.9; no longer C9.1, D12.A, D2.A, D3.C, R69.2, R78.1
- net N$45: now also C35.1, U$13.14; no longer D4.A, U8.7
- net N$46: now also C36.1, U$13.19; no longer D8.A, D9.C
- net N$47: now also C37.1, U$13.23; no longer D7.A, D8.C
- net N$48: now also C38.1, U$13.30; no longer D10.C, D9.A, R65.1, R75.1, U11.3
- net N$49: now also C39.1, U$13.35; no longer R75.2, U9.5, U9.7
- net N$50: now also C40.1, U$13.40; no longer C10.1, R73.2
- net N$51: now also C41.1, U$13.45; no longer D11.A, D12.C
- net N$52: now also C42.1, U$13.50; no longer D10.A, D11.C
- net N$53: now also C43.1, U$13.52; no longer R69.1, R72.2, U10.5
- net N$54: now also C44.1, U$13.53; no longer R78.2, U8.1
- net N$55: now also C45.1, U$13.55; no longer D7.C, R72.1, U10.7
- net N$56: now also C46.1, U$13.59; no longer D5.A, U10.1
- net N$57: now also C47.1, U$13.60; no longer C13.2, D17.A, D6.C, R90.2, U14.2
- net N$58: now also C48.1, U$13.62; no longer R97.2, R99.2, U15.3
- net N$59: now also C49.1, U$13.63; no longer R100.2, R81.1, U15.2
- net N$6: now also D19.A, D20.C, R13.2, R5.2, U10.3; no longer R12.1, U2.2
- net N$60: now also C19.2, U$13.5; no longer D19.C, R84.2, U14.5
- net N$61: now also R63.2, R65.2, U22.3; no longer R84.1, R85.2, U16.2
- net N$62: now also C21.2, U$13.10; no longer R86.1, U17.1, U17.5
- net N$63: now also C22.2, C35.2, U$13.13; no longer R86.2, R87.2, U17.2
- net N$64: now also C23.2, U$13.15; no longer D16.C, D6.A
- net N$65: now also C24.2, C36.2, U$13.18; no longer C13.1, D15.A, D16.A, D17.C, R89.2, R98.1
- net N$66: now also C25.2, C38.2, U$13.31; no longer D18.A, U14.7
- net N$67: now also C26.2, U$13.34; no longer D21.A, D22.C
- net N$69: now also C28.2, U$13.39; no longer D13.C, D22.A, R85.1, R95.1, U17.3
- net N$7: now also R14.2, R17.1, U10.2; no longer R13.2, R9.2, U2.6
- net N$70: now also C29.2, C40.2, U$13.41; no longer R95.2, U15.5, U15.7
- net N$71: now also R66.2, R67.1, U22.2; no longer C14.1, R93.2
- net N$72: now also C31.2, C41.2, U$13.46; no longer D14.A, D15.C
- net N$73: now also C32.2, U$13.49; no longer D13.A, D14.C
- net N$74: now also C43.2, U$13.51; no longer R89.1, R92.2, U16.5
- net N$75: now also C45.2, U$13.54; no longer R98.2, U14.1
- net N$76: now also C46.2, U$13.58; no longer D20.C, R92.1, U16.7
- net N$77: now also C48.2, U$13.61; no longer D19.A, U16.1
- net N$8: now also R36.1, R37.2, U11.5; no longer C1.1, R9.1, U2.7
- net N$9: now also C9.1, R35.2; no longer C2.1, R15.2
- net P0A: now also R25.1, R28.2, U$2.5; no longer R7.1, R8.2, U$1.5
- net P0A1: now also R56.1, R57.2, U$7.5; no longer R37.1, R38.2, U$2.5
- net P0A_0: now also R19.2, U$5.5; no longer R62.2, U$4.5
- net P0A_1: now also R39.1, U$6.5; no longer R74.1, U$5.5
- net P0B: now also R24.1, R34.1, U$2.7; no longer R14.1, R6.1, U$1.7
- net P0B1: now also R55.1, R81.1, U$7.7; no longer R36.1, R42.1, U$2.7
- net P0B_1: now also R38.1, U$6.7, U10.6; no longer R73.1, U$5.7, U9.6
- net P0W: now also R31.2, R32.1, R35.1, U$2.6; no longer R12.2, R13.1, R15.1, U$1.6
- net P0W1: now also R59.2, R60.1, R82.1, U$7.6; no longer R40.2, R41.1, R43.1, U$2.6
- net P0W_0: now also R14.1, U$5.6; no longer R80.1, U$4.6
- net PA0: now also R17.2, U$4.8, U10.1; no longer R61.2, U$3.8, U9.1
- net PA1: now also R29.2, U$4.7, U12.6; no longer R68.2, U$3.7, U11.6
- net PB0: now also R2.2, U$4.10, U9.3; no longer R76.2, U$3.10, U8.3
- net PB1: now also C7.2, U$4.5, U12.7; no longer C11.2, U$3.5, U11.7
- net RS: now also U$4.11; no longer U$3.11
- net RS1: now also U$10.11; no longer U$6.11
- net SCK: now also SCK1.1, U$10.2, U$11.2, U$12.2, U$14.2, U$15.2, U$18.2, U$19.2, U$2.2, U$20.2, U$21.2, U$3.2, U$4.2, U$5.2, U$6.2, U$7.2, U$9.2; no longer U$1.2
- net SCL: now also IC2.24, SCL1.1, U16.2, U19.2, U20.2, U26.14, U27.2, U39.2, U40.2, U8.2; no longer U6.2
- net SDA: now also IC2.23, SDA1.1, U16.3, U19.3, U20.3, U26.15, U27.3, U39.3, U40.3, U8.3; no longer U6.3
- net SDI/O: now also SDI/O1.1, U$10.3, U$11.3, U$12.3, U$14.3, U$15.3, U$18.3, U$19.3, U$2.3, U$20.3, U$21.3, U$3.3, U$4.3, U$5.3, U$6.3, U$7.3, U$9.3; no longer U$1.3
- net SHDN: now also U$4.12; no longer U$3.12
- net SHDN1: now also U$10.12; no longer U$6.12
- net VDD: now also 9VDD1.1, R124.1, R126.1, R151.1, R19.1, R68.1, R90.1, U$10.14, U$11.8, U$12.8, U$13.22, U$14.8, U$15.8, U$16.22, U$19.14, U$20.8, U$21.8, U$4.14, U$5.8, U$6.8, U$9.14, U10.8, U11.8, U12.8, U13.8, U15.8, U16.1, U19.1, U20.1, U20.4, U21.8, U22.8, U23.8, U24.8, U27.1, U27.4, U28.8, U29.8, U30.8, U31.8, U32.8, U39.1, U40.1, U40.4, U41.8, U42.8, U43.8, U44.8, U6.8, U7.1, U8.1, U8.4, U9.8; no longer U$14.22, U5.8
- net VREF: now also C16.2, C56.2, C71.2, C8.2, R1.1, R101.2, R106.1, R107.2, R108.2, R109.2, R137.1, R144.1, R145.1, R146.1, R152.2, R156.1, R157.1, R162.2, R189.1, R190.2, R191.2, R192.2, R2.1, R20.2, R21.1, R27.1, R29.1, R39.2, R43.1, R52.1, R53.1, R54.1, R61.1, R62.1, R63.1, R69.2, R73.1, R74.1, R79.2, R85.1, R91.2, R95.1, R96.1, U$11.7, U$14.7, U$18.8, U$20.7, U$3.8, U$5.7, U$7.8, U11.3, U11.6, U15.3, U15.5, U23.3, U23.6, U28.6, U28.7, U31.3, U31.6, U43.3, U43.6, U6.3, U6.5; no longer R28.1, R29.2, R30.2, R31.2, R33.1, R56.1, R57.2, R58.2, R59.2, U$1.8, U3.3, U3.5, U5.3, U5.5
- net VSS: now also GND1.1, GND3.1, GND4.1, GND8.1, R158.2, R33.2, R75.2, R97.2, U$10.4, U$11.4, U$12.4, U$14.4, U$15.4, U$19.4, U$20.4, U$21.4, U$6.4, U$9.4, U12.4, U16.4, U16.5, U16.9, U19.4, U19.5, U19.9, U20.5, U20.9, U21.4, U22.4, U23.4, U24.4, U27.5, U27.9, U29.4, U30.4, U31.4, U32.4, U39.4, U39.5, U39.9, U40.5, U40.9, U41.4, U42.4, U43.4, U44.4, U7.4, U8.5, U8.9; no longer R71.2, U$3.4, U6.4, U6.5, U6.9, U8.4
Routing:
- net VSS: track 1463.9 -> 580.9 mm, vias 9 -> 28
- net VREF: track 109.5 -> 671.5 mm, vias 8 -> 43
- net VDD: track 232.5 -> 513.8 mm, vias 5 -> 37
- net SDI/O: track 3.05 -> 246.5 mm, vias 0 -> 12
- net SCK: track 1.78 -> 229.4 mm, vias 0 -> 12
- net VSS1: track 206.2 -> 0.00 mm, vias 9 -> 0
- net VREF2: track 172.1 -> 0.00 mm, vias 8 -> 0
- net VREF1: track 172.1 -> 0.00 mm, vias 8 -> 0
- net EOUT0: track 163.8 -> 4.97 mm
- net VDD1: track 133.6 -> 0.00 mm, vias 7 -> 0
- net VDD2: track 133.6 -> 0.00 mm, vias 7 -> 0
- net EOUT1: track 132.7 -> 5.55 mm
- net SCK2: track 109.0 -> 0.00 mm, vias 2 -> 0
- net GND: track 60.1 -> 166.3 mm, vias 8 -> 15
- net N$40: track 105.8 -> 3.63 mm
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- removed copper zone on layer 2, net GND
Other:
- board size 179 x 79.7 mm -> 121.9 x 109.2 mm
